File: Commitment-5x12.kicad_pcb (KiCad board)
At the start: 2 copper layers, 234.4 x 118.4 mm, 97 parts, among them J1 Conn_01x13, J2 Conn_01x13, J3 Conn_01x03, J4 Conn_01x04, J5 Conn_01x04, SW1 OS102011MS2QN1, SW2 RotaryEncoder

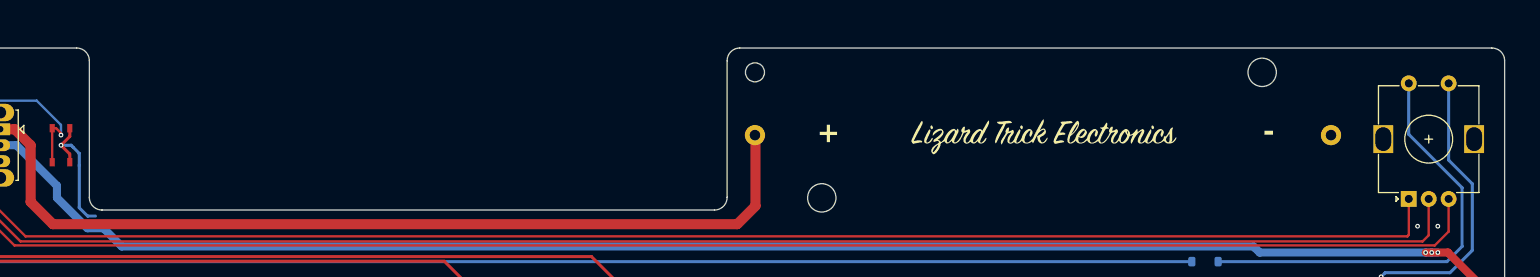
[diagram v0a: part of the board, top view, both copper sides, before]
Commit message: working toward rev 1
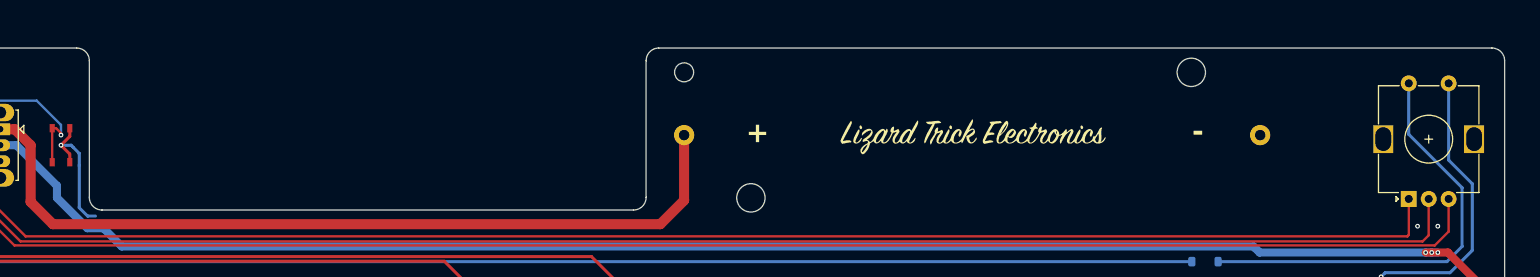
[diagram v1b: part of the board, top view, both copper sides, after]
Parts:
- moved BAT1 8.89 mm to (190.5, 35.6)
- moved G*** 8.89 mm to (190.5, 35.6)
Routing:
- net Net-(BAT1-+): track 113.7 -> 104.3 mm
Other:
- outline, holes or cut-outs redrawn
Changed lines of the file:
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@@
 		(pad_to_mask_clearance 0)
 		(allow_soldermask_bridges_in_footprints no)
-		(grid_origin 35.56 62.23)
+		(grid_origin 38.1 57.15)
 		(pcbplotparams
 			(layerselection 0x00010fc_ffffffff)
@@
 		(tags "Cherry MX keyswitch 2.00u PCB")
 		(property "Reference" "M1"
-			(at -2.54 -2.794 360)
+			(at -2.54 -2.794 0)
 			(layer "F.SilkS")
 			(hide yes)
@@
 		)
 		(property "Value" "~"
-			(at -2.54 12.954 360)
+			(at -2.54 12.954 0)
 			(layer "F.Fab")
 			(effects
@@
 		)
 		(fp_text user "${REFERENCE}"
-			(at -2.54 -2.794 360)
+			(at -2.54 -2.794 0)
 			(layer "F.Fab")
 			(effects
@@
 	(footprint "lizard_libs:Lizard Text Logo"
 		(layer "F.Cu")
-		(at 199.39 35.56)
+		(at 190.5 35.56)
 		(property "Reference" "G***"
 			(at 0 2.54 0)
@@
 		(tags "Cherry MX keyswitch 2.00u PCB")
 		(property "Reference" "M2"
-			(at -2.54 -2.794 360)
+			(at -2.54 -2.794 0)
 			(layer "F.SilkS")
 			(hide yes)
@@
 		)
 		(property "Value" "~"
-			(at -2.54 12.954 360)
+			(at -2.54 12.954 0)
 			(layer "F.Fab")
 			(effects
@@
 		)
 		(fp_text user "${REFERENCE}"
-			(at -2.54 -2.794 360)
+			(at -2.54 -2.794 0)
 			(layer "F.Fab")
 			(effects
@@
 	(footprint "lizard_libs:Keystone 1043 18650"
 		(layer "F.Cu")
-		(at 199.39 35.56 180)
+		(at 190.5 35.56 180)
 		(property "Reference" "BAT1"
 			(at 0 -2.54 180)
@@
 	)
 	(gr_arc
-		(start 159.766 26.2255)
-		(mid 160.230968 25.102968)
-		(end 161.3535 24.638)
+		(start 149.606 26.2255)
+		(mid 150.070968 25.102968)
+		(end 151.1935 24.638)
 		(stroke
 			(width 0.05)
@@
 	)
 	(gr_line
-		(start 159.766 26.2255)
-		(end 159.766 43.3705)
+		(start 149.606 26.2255)
+		(end 149.606 43.3705)
 		(stroke
 			(width 0.05)
@@
 	)
 	(gr_line
-		(start 158.1785 44.958)
+		(start 148.0185 44.958)
 		(end 81.3435 44.958)
 		(stroke
@@
 	)
 	(gr_arc
-		(start 159.766 43.3705)
-		(mid 159.301032 44.493032)
-		(end 158.1785 44.958)
+		(start 149.606 43.3705)
+		(mid 149.141032 44.493032)
+		(end 148.0185 44.958)
 		(stroke
 			(width 0.05)
@@
 	)
 	(gr_line
-		(start 161.3535 24.638)
+		(start 151.1935 24.638)
 		(end 255.7145 24.638)
 		(stroke
@@
 	)
 	(gr_text "+"
-		(at 172.466 35.433 180)
+		(at 163.576 35.433 180)
 		(layer "F.SilkS")
 		(effects
@@
 	)
 	(gr_text "-"
-		(at 227.711 35.433 180)
+		(at 218.821 35.433 180)
 		(layer "F.SilkS")
 		(effects
@@
 	)
 	(segment
-		(start 70.39 34.83)
-		(end 72.39 36.83)
-		(width 1.27)
-		(layer "F.Cu")
-		(net 1)
-	)
-	(segment
-		(start 163.322 44.45)
-		(end 163.322 35.6235)
+		(start 68.58 34.83)
+		(end 70.39 34.83)
 		(width 1.27)
 		(layer "F.Cu")
@@
 	(segment
 		(start 75.184 46.736)
-		(end 161.036 46.736)
+		(end 151.384 46.736)
 		(width 1.27)
 		(layer "F.Cu")
@@
 	)
 	(segment
-		(start 163.322 35.6235)
-		(end 163.2585 35.56)
+		(start 154.3685 43.7515)
+		(end 154.3685 35.56)
 		(width 1.27)
 		(layer "F.Cu")
@@
 	)
 	(segment
-		(start 68.58 34.83)
-		(end 70.39 34.83)
+		(start 70.39 34.83)
+		(end 72.39 36.83)
 		(width 1.27)
 		(layer "F.Cu")
@@
 	)
 	(segment
-		(start 161.036 46.736)
-		(end 163.322 44.45)
+		(start 151.384 46.736)
+		(end 154.3685 43.7515)
 		(width 1.27)
 		(layer "F.Cu")
@@
 		)
 	)
+	(group ""
+		(members "3122b99c-ad25-44f4-953b-640c3fc964a2" "711c629b-a350-407e-8104-c2bea098a2da"
+			"d03c237c-e164-42e6-be8a-686f8292c659"
+		)
+	)
